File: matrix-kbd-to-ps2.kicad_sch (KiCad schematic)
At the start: 14 parts, among them J1 CN13-CN14, J2 PS/2 - Mini-Din6, U1 PIC24FJ64GB002, U2 AMS1117

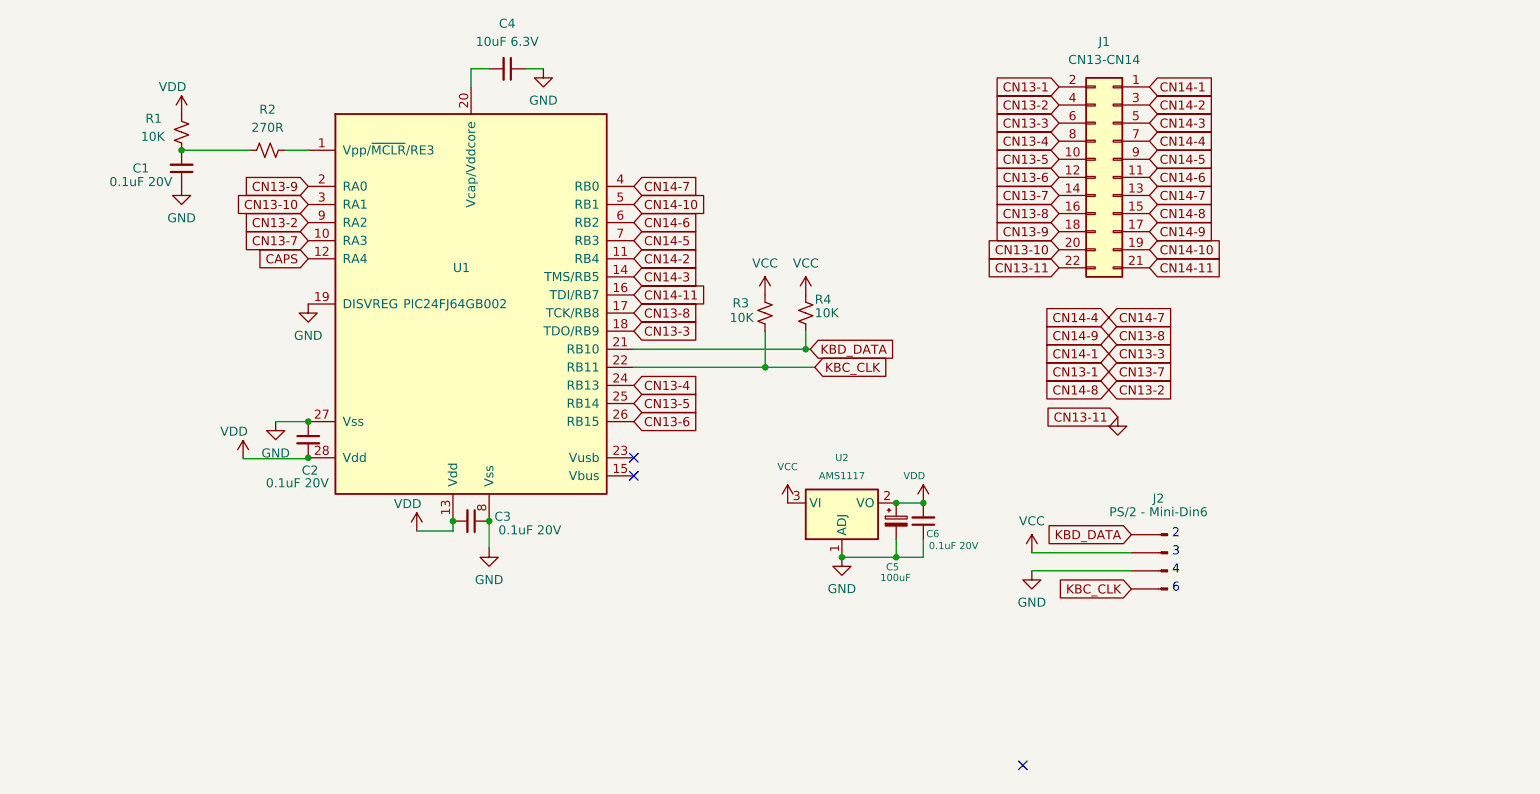
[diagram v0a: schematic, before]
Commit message: Revision 1
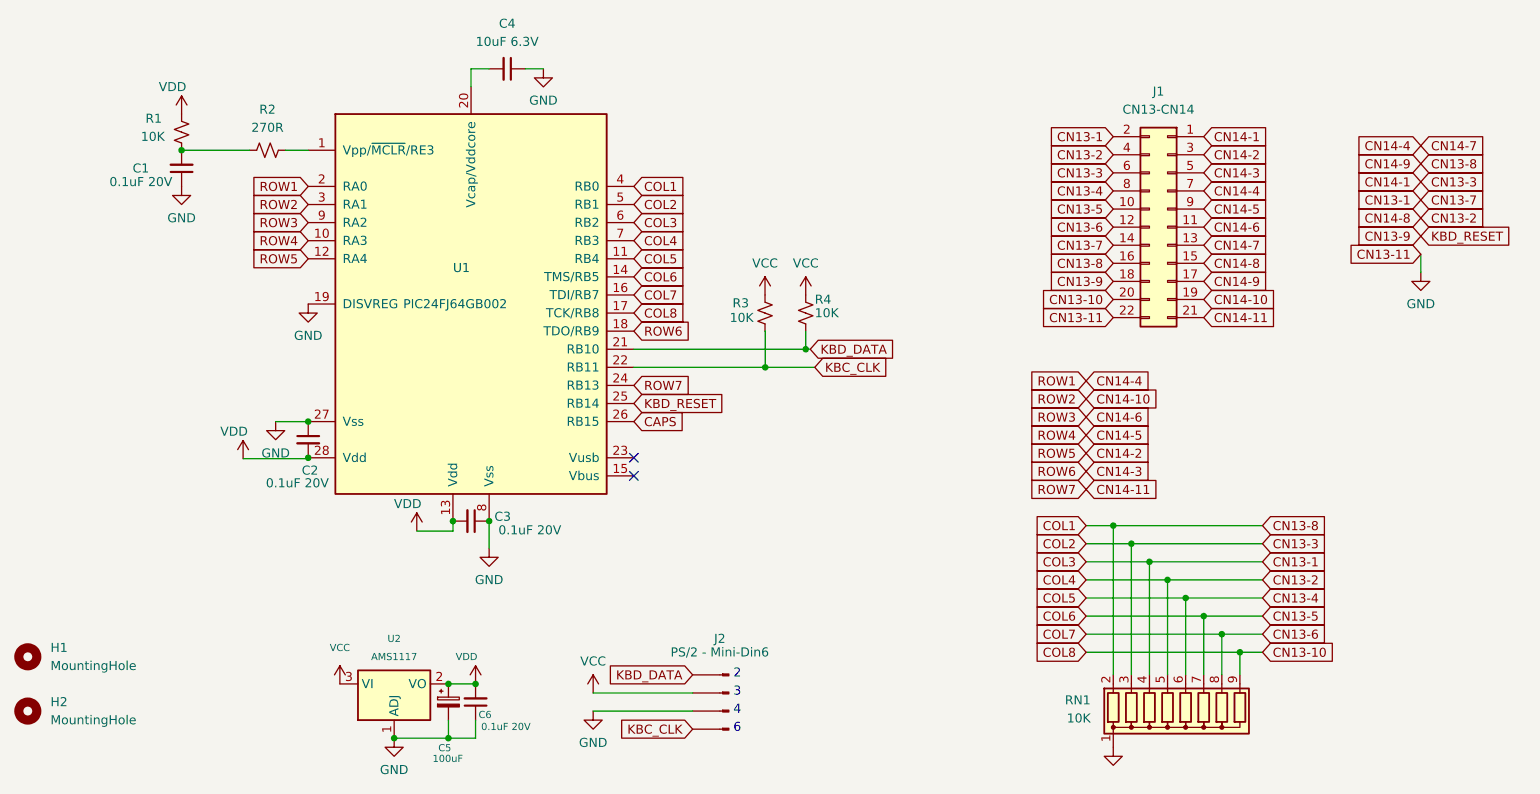
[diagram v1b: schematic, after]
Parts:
- added H1, H2: MountingHole, MountingHole:MountingHole_2.5mm, symbol Mechanical:MountingHole
- added RN1: 10K, Resistor_THT:R_Array_SIP9, symbol Device:R_Network08
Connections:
- net CAPS: now also U1.26 (RB15); no longer U1.12 (RA4)
- net CN13-1: now also U1.6 (RB2), RN1.4 (R3); no longer U1.10 (RA3)
- net CN13-10: now also U1.17 (TCK/RB8), RN1.9 (R8); no longer U1.3 (RA1)
- net CN13-2: now also U1.7 (RB3), RN1.5 (R4); no longer U1.9 (RA2)
- net CN13-3: now also U1.5 (RB1), RN1.3 (R2); no longer U1.18 (TDO/RB9)
- net CN13-4: now also U1.11 (RB4), RN1.6 (R5); no longer U1.24 (RB13)
- net CN13-5: now also U1.14 (TMS/RB5), RN1.7 (R6); no longer U1.25 (RB14)
- net CN13-6: now also U1.16 (TDI/RB7), RN1.8 (R7); no longer U1.26 (RB15)
- net CN13-8: now also U1.4 (RB0), RN1.2 (R1); no longer U1.17 (TCK/RB8)
- net CN13-9: now also U1.25 (RB14); no longer U1.2 (RA0)
- net CN14-10: now also U1.3 (RA1); no longer U1.5 (RB1)
- net CN14-11: now also U1.24 (RB13); no longer U1.16 (TDI/RB7)
- net CN14-2: now also U1.12 (RA4); no longer U1.11 (RB4)
- net CN14-3: now also U1.18 (TDO/RB9); no longer U1.14 (TMS/RB5)
- net CN14-4: now also U1.2 (RA0); no longer U1.4 (RB0)
- net CN14-5: now also U1.10 (RA3); no longer U1.7 (RB3)
- net CN14-6: now also U1.9 (RA2); no longer U1.6 (RB2)
- net GND: now also RN1.1 (common)
- no-connect marks 3 -> 2
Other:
- moved on the sheet: C5, C6, J1, J2, U2
